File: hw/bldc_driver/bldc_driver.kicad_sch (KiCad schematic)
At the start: 25 parts, among them U1 CH32V30xRxTx, U14 SN65HVD230, U8 TPS54202DDC

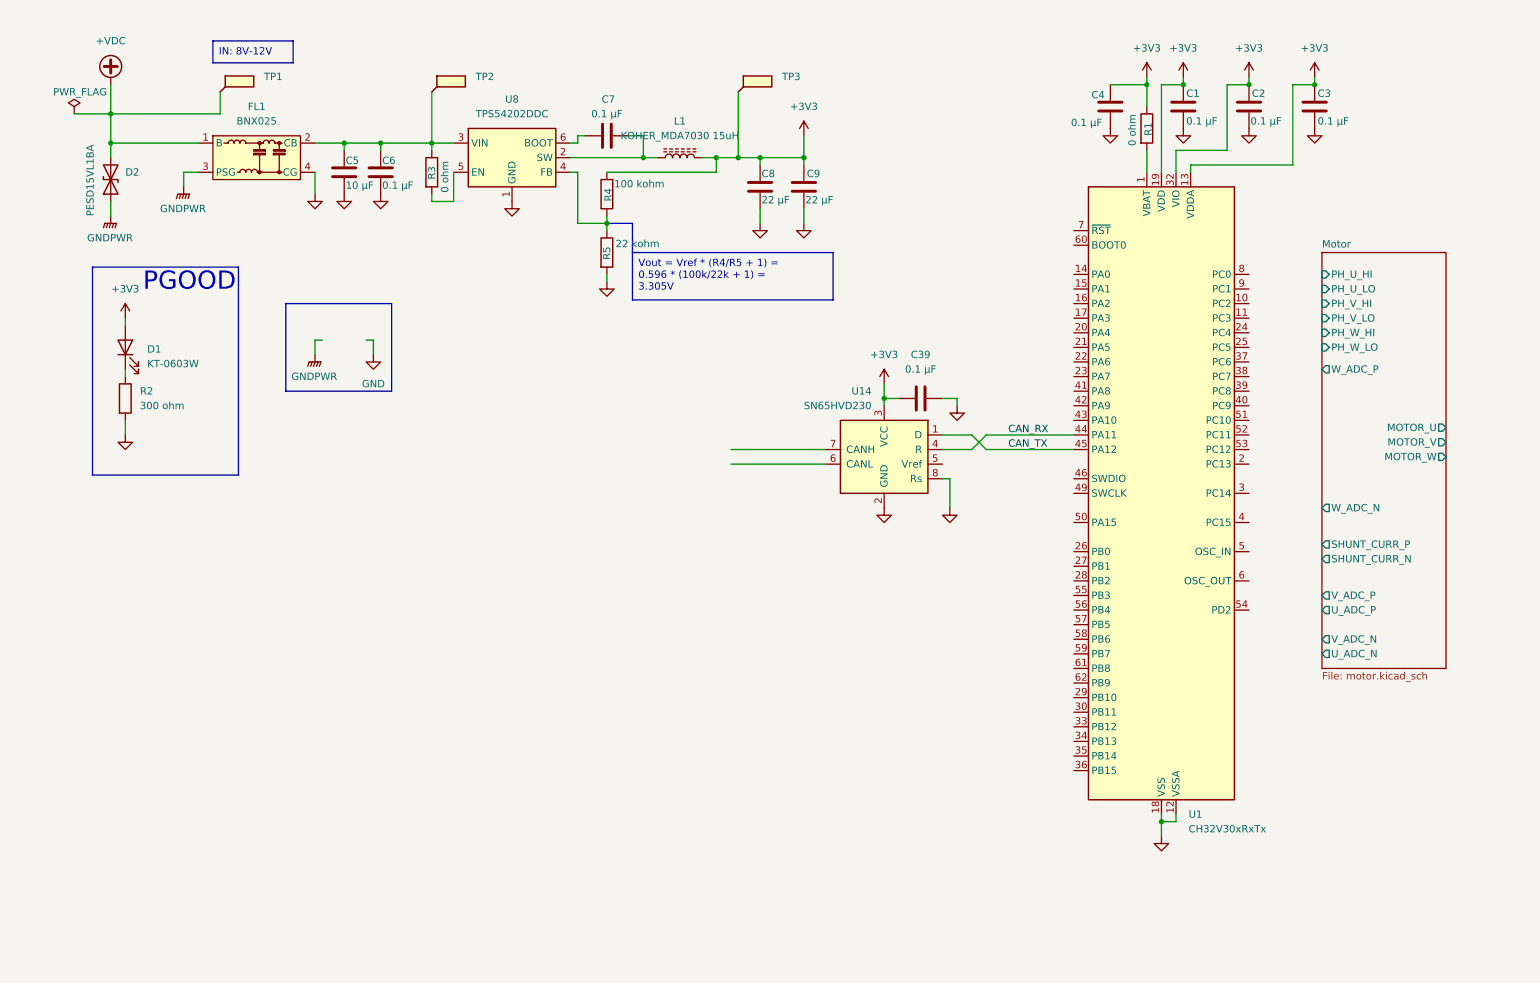
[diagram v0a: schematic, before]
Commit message: feat: add CNCs
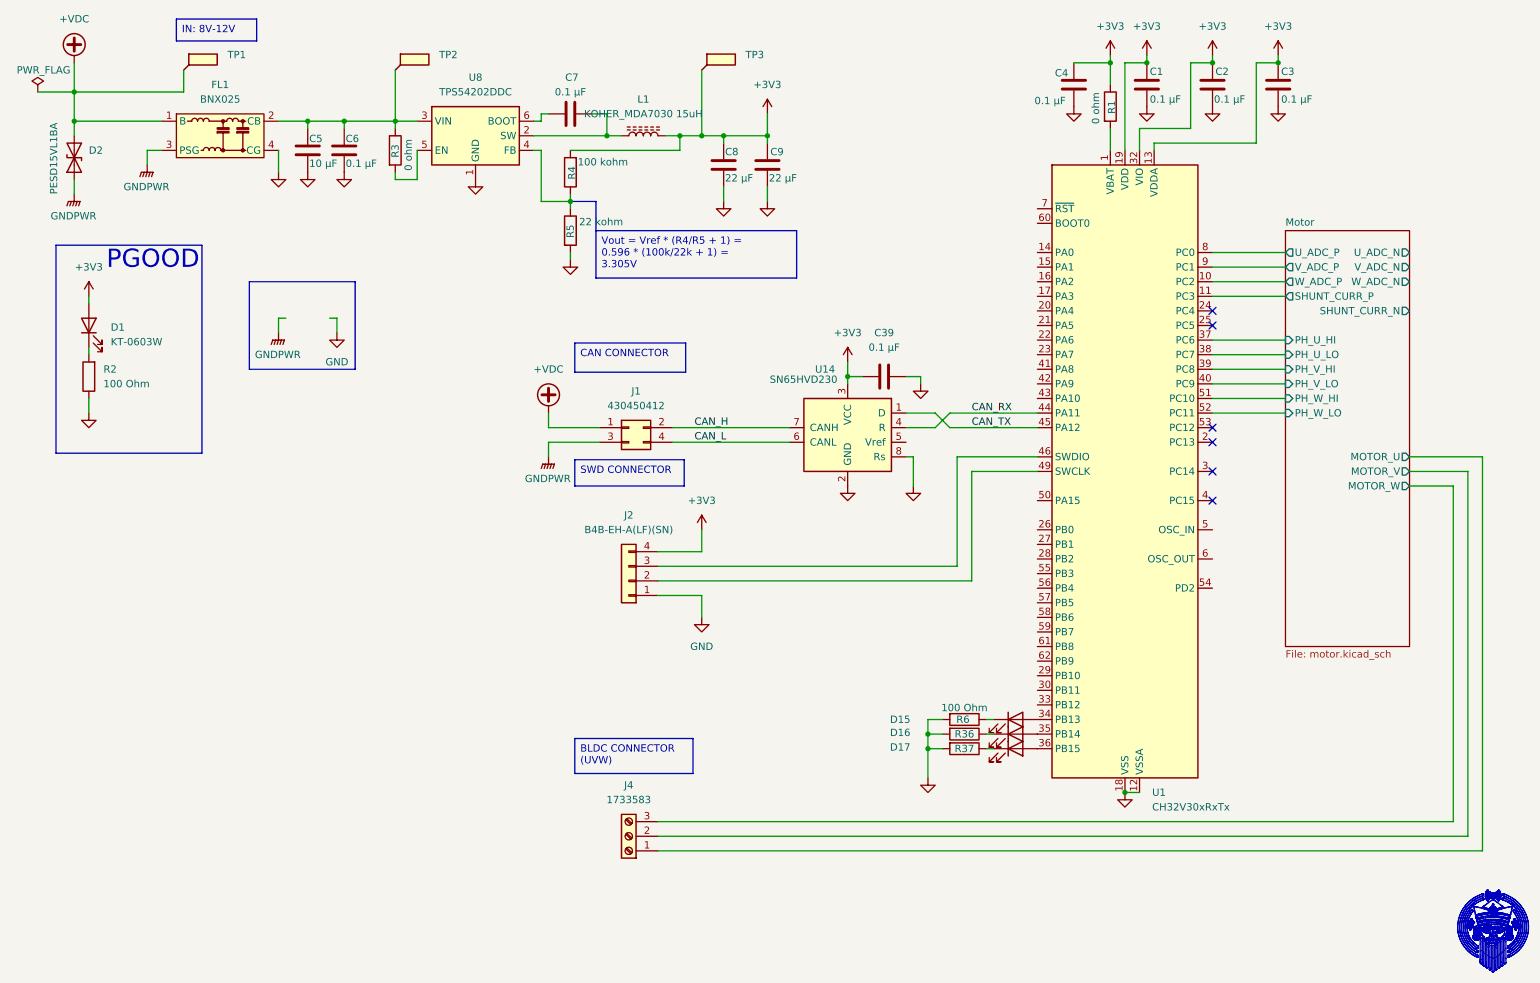
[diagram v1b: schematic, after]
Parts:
- removed R2: 300 ohm, Resistor_SMD:R_0603_1608Metric_Pad0.98x0.95mm_HandSolder, symbol #inventree:RC0603FR-07300RL
- added D15, D16, D17: KT-0603W, LED_SMD:LED_0603_1608Metric_Pad1.05x0.95mm_HandSolder, symbol Device:LED
- added J1: 430450412, Connector_Molex:Molex_Micro-Fit_3.0_43045-0412_2x02_P3.00mm_Vertical, symbol Connector_Generic:Conn_02x02_Odd_Even
- added J2: B4B-EH-A(LF)(SN), Connector_JST:JST_EH_B4B-EH-A_1x04_P2.50mm_Vertical, symbol Connector_Generic:Conn_01x04
- added J4: 1733583, TerminalBlock_Phoenix:TerminalBlock_Phoenix_MKDS-1,5-3-5.08_1x03_P5.08mm_Horizontal, symbol Connector:Screw_Terminal_01x03
- added R2, R36, R37, R6: 100 Ohm, Resistor_SMD:R_0603_1608Metric_Pad0.98x0.95mm_HandSolder, symbol Device:R
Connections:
- net +3V3: now also J2.4 (Pin_4)
- net +VDC: now also J1.1 (Pin_1)
- net GND: now also J2.1 (Pin_1), R2.1, R36.2, R37.2, R6.2
- net GNDPWR: now also J1.3 (Pin_3)
- net Motor/MOTOR_U: now also J4.1 (Pin_1)
- net Motor/MOTOR_V: now also J4.2 (Pin_2)
- net Motor/MOTOR_W: now also J4.3 (Pin_3)
- net Motor/PH_U_HI: now also U1.37 (PC6)
- net Motor/PH_U_LO: now also U1.38 (PC7)
- net Motor/PH_V_HI: now also U1.39 (PC8)
- net Motor/PH_V_LO: now also U1.40 (PC9)
- net Motor/PH_W_HI: now also U1.51 (PC10)
- net Motor/PH_W_LO: now also U1.52 (PC11)
- net Motor/SHUNT_CURR_P: now also U1.11 (PC3)
- net Motor/U_ADC_P: now also U1.8 (PC0)
- net Motor/V_ADC_P: now also U1.9 (PC1)
- net Motor/W_ADC_P: now also U1.10 (PC2)
- net at U1.34 (PB13): now also D15.2 (A)
- net at U1.35 (PB14): now also D16.2 (A)
- net at U1.36 (PB15): now also D17.2 (A)
- net at U1.46 (SWDIO): now also J2.3 (Pin_3)
- net at U1.49 (SWCLK): now also J2.2 (Pin_2)
- net at D1.1 (K): now also R2.2
- net CAN_L: now reaches U14.6 (CANL)
- net CAN_L: now also J1.4 (Pin_4)
- net CAN_H: now reaches U14.7 (CANH)
- net CAN_H: now also J1.2 (Pin_2)
- new net: D17.1 (K), R37.1
- new net: D15.1 (K), R6.1
- new net: D16.1 (K), R36.1
- no-connect marks 0 -> 6
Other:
- moved on the sheet: C1, C2, C3, C39, C4, C5, C6, C7, C8, C9, D1, D2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
